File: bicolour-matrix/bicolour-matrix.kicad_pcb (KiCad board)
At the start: 2 copper layers, 136.8 x 33.5 mm, 52 parts, among them J1 Conn_01x04_Pin, J2 Conn_01x04_Pin, U1 HT16K33A-28SSOP, U2 HT16K33A-28SSOP, U3 HT16K33A-28SSOP, U4 HT16K33A-28SSOP

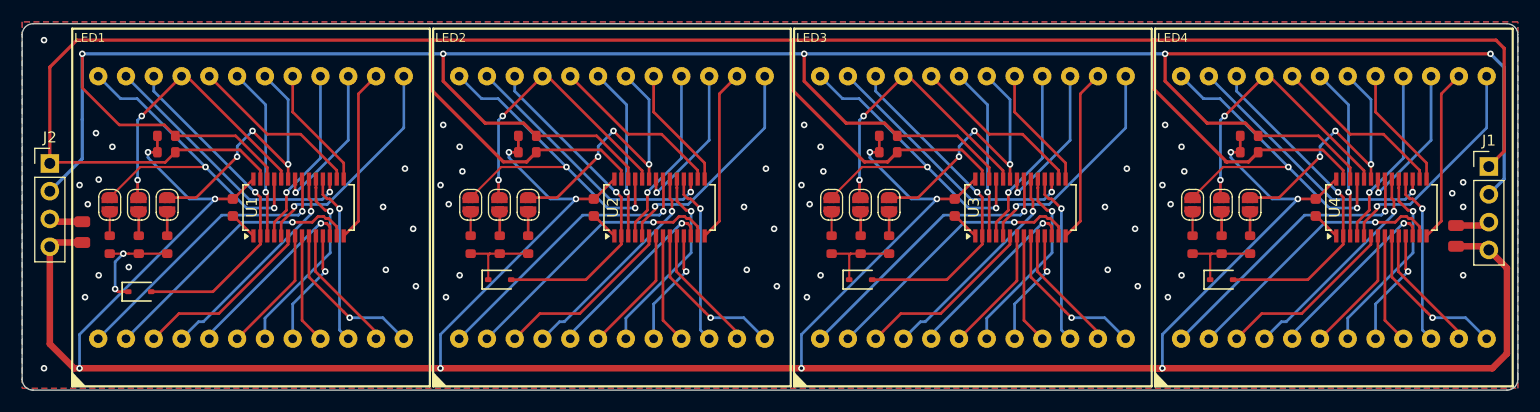
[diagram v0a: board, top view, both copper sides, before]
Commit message: feat: all changes
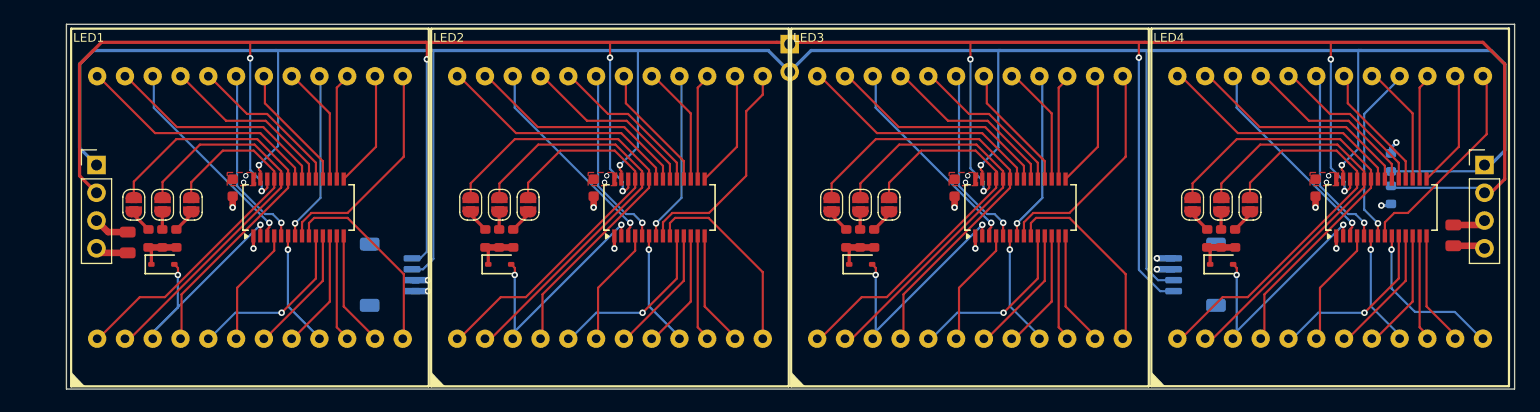
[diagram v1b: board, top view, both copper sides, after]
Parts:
- removed R12, R16, R17, R6, R7, R8: 4.7kΩ, PCM_JLCPCB:R_0603
- added J3: Conn_01x04_Socket, Connector_JST:JST_SH_SM04B-SRSS-TB_1x04-1MP_P1.00mm_Horizontal, B.Cu at (191.8, 94.0)
- added J4: Conn_01x04_Socket, Connector_JST:JST_SH_SM04B-SRSS-TB_1x04-1MP_P1.00mm_Horizontal, B.Cu at (118.2, 94.0)
- added J5: Conn_01x02_Socket, Connector_PinSocket_2.54mm:PinSocket_1x02_P2.54mm_Vertical, B.Cu at (154.7, 72.9)
- C2, C3, C4, C5: value 1uF -> 100nF
- R1, R2: value 4.7kΩ -> 10kΩ; footprint PCM_JLCPCB:R_0603 -> Resistor_SMD:R_0603_1608Metric; moved to B.Cu
- moved R1 79.1 mm to (209.7, 86.7), turned to 90 degrees
- moved R2 79.0 mm to (209.7, 83.7), turned to -90 degrees
- moved J2 4.27 mm to (91.3, 83.9)
- moved C6 4.26 mm to (94.2, 91.0)
- moved R11 3.59 mm to (96.0, 90.6)
- moved D1 3.27 mm to (97.4, 93.0)
- moved R9 2.23 mm to (97.3, 90.6)
- moved JP1 2.20 mm to (97.3, 87.5)
- moved JP2 2.20 mm to (100.0, 87.5)
- moved JP3 2.20 mm to (94.7, 87.5)
- moved C2 1.80 mm to (103.7, 86.0)
- moved C3 1.80 mm to (136.8, 86.0)
- moved C4 1.80 mm to (169.8, 86.0)
- moved C5 1.80 mm to (202.8, 86.0)
- moved R15 1.48 mm to (162.4, 90.6)
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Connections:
- net Net-(LED1-K8) renamed /Matrix 1/C7
- net Net-(LED2-K8) renamed /Matrix 2/C7
- net Net-(LED3-K8) renamed /Matrix 3/C7
- net Net-(LED4-K8) renamed /Matrix 4/C7
- D1 pad 2: Net-(LED1-K1) -> /Matrix 1/C0
- D2 pad 2: Net-(LED2-K1) -> /Matrix 2/C0
- D3 pad 2: Net-(LED3-K1) -> /Matrix 3/C0
- D4 pad 2: Net-(LED4-K1) -> /Matrix 4/C0
- J1 pad 1: /Matrix 1/SDA -> /SDA
- J1 pad 2: /Matrix 1/SCL -> /SCL
- J2 pad 1: /Matrix 1/SDA -> /SDA
- J2 pad 2: /Matrix 1/SCL -> /SCL
- JP1 pad 2: /Matrix 1/A1-1 -> /Matrix 1/R1
- JP10 pad 2: /Matrix 4/A2-1 -> /Matrix 4/R2
- JP11 pad 2: /Matrix 4/A1-1 -> /Matrix 4/R1
- JP12 pad 2: /Matrix 4/A0-1 -> /Matrix 4/R0
- JP2 pad 2: /Matrix 1/A0-1 -> /Matrix 1/R0
- JP3 pad 2: /Matrix 1/A2-1 -> /Matrix 1/R2
- JP4 pad 2: /Matrix 2/A2-1 -> /Matrix 2/R2
- JP5 pad 2: /Matrix 2/A1-1 -> /Matrix 2/R1
- JP6 pad 2: /Matrix 2/A0-1 -> /Matrix 2/R0
- JP7 pad 2: /Matrix 3/A2-1 -> /Matrix 3/R2
- JP8 pad 2: /Matrix 3/A1-1 -> /Matrix 3/R1
- JP9 pad 2: /Matrix 3/A0-1 -> /Matrix 3/R0
- LED1 pad 1: Net-(LED1-A9) -> /Matrix 1/R0
- LED1 pad 10: Net-(LED1-A15) -> /Matrix 1/R12
- LED1 pad 11: Net-(LED1-A16) -> /Matrix 1/R11
- LED1 pad 13: Net-(LED1-K4) -> /Matrix 1/C6
- LED1 pad 14: Net-(LED1-A8) -> /Matrix 1/R10
- LED1 pad 15: Net-(LED1-A7) -> /Matrix 1/R9
- LED1 pad 16: Net-(LED1-K3) -> /Matrix 1/C5
- LED1 pad 17: Net-(LED1-A6) -> /Matrix 1/R8
- LED1 pad 18: /Matrix 1/A0-1 -> /Matrix 1/R7
- LED1 pad 19: Net-(LED1-K2) -> /Matrix 1/C3
- LED1 pad 2: Net-(LED1-A10) -> /Matrix 1/R1
- LED1 pad 20: Net-(LED1-A4) -> /Matrix 1/R6
- LED1 pad 21: /Matrix 1/A1-1 -> /Matrix 1/R5
- LED1 pad 22: Net-(LED1-K1) -> /Matrix 1/C1
- LED1 pad 23: Net-(LED1-A2) -> /Matrix 1/R4
- LED1 pad 24: /Matrix 1/A2-1 -> /Matrix 1/R3
- LED1 pad 3: Net-(LED1-K5) -> /Matrix 1/C0
- LED1 pad 4: Net-(LED1-A11) -> /Matrix 1/R2
- LED1 pad 5: Net-(LED1-A12) -> /Matrix 1/R15
- LED1 pad 6: Net-(LED1-K6) -> /Matrix 1/C2
- LED1 pad 7: Net-(LED1-A13) -> /Matrix 1/R14
- LED1 pad 8: Net-(LED1-A14) -> /Matrix 1/R13
- LED1 pad 9: Net-(LED1-K7) -> /Matrix 1/C4
- LED2 pad 1: Net-(LED2-A9) -> /Matrix 2/R0
- LED2 pad 10: Net-(LED2-A15) -> /Matrix 2/R12
- LED2 pad 11: Net-(LED2-A16) -> /Matrix 2/R11
- LED2 pad 13: Net-(LED2-K4) -> /Matrix 2/C6
- LED2 pad 14: Net-(LED2-A8) -> /Matrix 2/R10
- LED2 pad 15: Net-(LED2-A7) -> /Matrix 2/R9
- LED2 pad 16: Net-(LED2-K3) -> /Matrix 2/C5
- LED2 pad 17: Net-(LED2-A6) -> /Matrix 2/R8
- LED2 pad 18: /Matrix 2/A0-1 -> /Matrix 2/R7
- LED2 pad 19: Net-(LED2-K2) -> /Matrix 2/C3
- LED2 pad 2: Net-(LED2-A10) -> /Matrix 2/R1
- LED2 pad 20: Net-(LED2-A4) -> /Matrix 2/R6
- LED2 pad 21: /Matrix 2/A1-1 -> /Matrix 2/R5
- LED2 pad 22: Net-(LED2-K1) -> /Matrix 2/C1
- LED2 pad 23: Net-(LED2-A2) -> /Matrix 2/R4
- LED2 pad 24: /Matrix 2/A2-1 -> /Matrix 2/R3
- LED2 pad 3: Net-(LED2-K5) -> /Matrix 2/C0
- LED2 pad 4: Net-(LED2-A11) -> /Matrix 2/R2
- LED2 pad 5: Net-(LED2-A12) -> /Matrix 2/R15
- LED2 pad 6: Net-(LED2-K6) -> /Matrix 2/C2
- LED2 pad 7: Net-(LED2-A13) -> /Matrix 2/R14
- LED2 pad 8: Net-(LED2-A14) -> /Matrix 2/R13
- LED2 pad 9: Net-(LED2-K7) -> /Matrix 2/C4
- LED3 pad 1: Net-(LED3-A9) -> /Matrix 3/R0
- LED3 pad 10: Net-(LED3-A15) -> /Matrix 3/R12
- LED3 pad 11: Net-(LED3-A16) -> /Matrix 3/R11
- LED3 pad 13: Net-(LED3-K4) -> /Matrix 3/C6
- LED3 pad 14: Net-(LED3-A8) -> /Matrix 3/R10
- LED3 pad 15: Net-(LED3-A7) -> /Matrix 3/R9
- LED3 pad 16: Net-(LED3-K3) -> /Matrix 3/C5
- LED3 pad 17: Net-(LED3-A6) -> /Matrix 3/R8
- LED3 pad 18: /Matrix 3/A0-1 -> /Matrix 3/R7
- LED3 pad 19: Net-(LED3-K2) -> /Matrix 3/C3
- LED3 pad 2: Net-(LED3-A10) -> /Matrix 3/R1
- LED3 pad 20: Net-(LED3-A4) -> /Matrix 3/R6
- LED3 pad 21: /Matrix 3/A1-1 -> /Matrix 3/R5
- LED3 pad 22: Net-(LED3-K1) -> /Matrix 3/C1
- LED3 pad 23: Net-(LED3-A2) -> /Matrix 3/R4
- LED3 pad 24: /Matrix 3/A2-1 -> /Matrix 3/R3
- LED3 pad 3: Net-(LED3-K5) -> /Matrix 3/C0
- LED3 pad 4: Net-(LED3-A11) -> /Matrix 3/R2
- LED3 pad 5: Net-(LED3-A12) -> /Matrix 3/R15
- LED3 pad 6: Net-(LED3-K6) -> /Matrix 3/C2
- LED3 pad 7: Net-(LED3-A13) -> /Matrix 3/R14
- LED3 pad 8: Net-(LED3-A14) -> /Matrix 3/R13
- LED3 pad 9: Net-(LED3-K7) -> /Matrix 3/C4
- LED4 pad 1: Net-(LED4-A9) -> /Matrix 4/R0
- LED4 pad 10: Net-(LED4-A15) -> /Matrix 4/R12
- LED4 pad 11: Net-(LED4-A16) -> /Matrix 4/R11
- LED4 pad 13: Net-(LED4-K4) -> /Matrix 4/C6
- LED4 pad 14: Net-(LED4-A8) -> /Matrix 4/R10
- LED4 pad 15: Net-(LED4-A7) -> /Matrix 4/R9
- LED4 pad 16: Net-(LED4-K3) -> /Matrix 4/C5
- LED4 pad 17: Net-(LED4-A6) -> /Matrix 4/R8
- LED4 pad 18: /Matrix 4/A0-1 -> /Matrix 4/R7
- LED4 pad 19: Net-(LED4-K2) -> /Matrix 4/C3
- LED4 pad 2: Net-(LED4-A10) -> /Matrix 4/R1
- LED4 pad 20: Net-(LED4-A4) -> /Matrix 4/R6
- LED4 pad 21: /Matrix 4/A1-1 -> /Matrix 4/R5
- LED4 pad 22: Net-(LED4-K1) -> /Matrix 4/C1
- LED4 pad 23: Net-(LED4-A2) -> /Matrix 4/R4
- LED4 pad 24: /Matrix 4/A2-1 -> /Matrix 4/R3
- LED4 pad 3: Net-(LED4-K5) -> /Matrix 4/C0
- LED4 pad 4: Net-(LED4-A11) -> /Matrix 4/R2
- LED4 pad 5: Net-(LED4-A12) -> /Matrix 4/R15
- LED4 pad 6: Net-(LED4-K6) -> /Matrix 4/C2
- LED4 pad 7: Net-(LED4-A13) -> /Matrix 4/R14
- LED4 pad 8: Net-(LED4-A14) -> /Matrix 4/R13
- LED4 pad 9: Net-(LED4-K7) -> /Matrix 4/C4
- R1 pad 2: /Matrix 1/SDA -> /SCL
- R2 pad 2: /Matrix 1/SCL -> /SDA
- U1 pad 10: Net-(LED1-A16) -> /Matrix 1/R15
- U1 pad 11: Net-(LED1-A14) -> /Matrix 1/R14
- U1 pad 12: Net-(LED1-A12) -> /Matrix 1/R13
- U1 pad 13: Net-(LED1-A10) -> /Matrix 1/R12
- U1 pad 14: Net-(LED1-A8) -> /Matrix 1/R11
- U1 pad 15: Net-(LED1-A6) -> /Matrix 1/R10
- U1 pad 16: Net-(LED1-A4) -> /Matrix 1/R9
- U1 pad 17: Net-(LED1-A2) -> /Matrix 1/R8
- U1 pad 18: Net-(LED1-A15) -> /Matrix 1/R7
- U1 pad 19: Net-(LED1-A13) -> /Matrix 1/R6
- U1 pad 2: Net-(LED1-K1) -> /Matrix 1/C0
- U1 pad 20: Net-(LED1-A11) -> /Matrix 1/R5
- U1 pad 21: Net-(LED1-A9) -> /Matrix 1/R4
- U1 pad 22: Net-(LED1-A7) -> /Matrix 1/R3
- U1 pad 23: /Matrix 1/A0-1 -> /Matrix 1/R2
- U1 pad 24: /Matrix 1/A1-1 -> /Matrix 1/R1
- U1 pad 25: /Matrix 1/A2-1 -> /Matrix 1/R0
- U1 pad 26: /Matrix 1/SCL -> /SCL
- U1 pad 27: /Matrix 1/SDA -> /SDA
- U1 pad 3: Net-(LED1-K2) -> /Matrix 1/C1
- U1 pad 4: Net-(LED1-K3) -> /Matrix 1/C2
- U1 pad 5: Net-(LED1-K4) -> /Matrix 1/C3
- U1 pad 6: Net-(LED1-K5) -> /Matrix 1/C4
- U1 pad 7: Net-(LED1-K6) -> /Matrix 1/C5
- U1 pad 8: Net-(LED1-K7) -> /Matrix 1/C6
- U2 pad 10: Net-(LED2-A16) -> /Matrix 2/R15
- U2 pad 11: Net-(LED2-A14) -> /Matrix 2/R14
- U2 pad 12: Net-(LED2-A12) -> /Matrix 2/R13
- U2 pad 13: Net-(LED2-A10) -> /Matrix 2/R12
- U2 pad 14: Net-(LED2-A8) -> /Matrix 2/R11
- U2 pad 15: Net-(LED2-A6) -> /Matrix 2/R10
- U2 pad 16: Net-(LED2-A4) -> /Matrix 2/R9
- U2 pad 17: Net-(LED2-A2) -> /Matrix 2/R8
- U2 pad 18: Net-(LED2-A15) -> /Matrix 2/R7
- U2 pad 19: Net-(LED2-A13) -> /Matrix 2/R6
- U2 pad 2: Net-(LED2-K1) -> /Matrix 2/C0
- U2 pad 20: Net-(LED2-A11) -> /Matrix 2/R5
- U2 pad 21: Net-(LED2-A9) -> /Matrix 2/R4
- U2 pad 22: Net-(LED2-A7) -> /Matrix 2/R3
- U2 pad 23: /Matrix 2/A0-1 -> /Matrix 2/R2
- U2 pad 24: /Matrix 2/A1-1 -> /Matrix 2/R1
- U2 pad 25: /Matrix 2/A2-1 -> /Matrix 2/R0
- U2 pad 26: /Matrix 1/SCL -> /SCL
- U2 pad 27: /Matrix 1/SDA -> /SDA
- U2 pad 3: Net-(LED2-K2) -> /Matrix 2/C1
- U2 pad 4: Net-(LED2-K3) -> /Matrix 2/C2
- U2 pad 5: Net-(LED2-K4) -> /Matrix 2/C3
- U2 pad 6: Net-(LED2-K5) -> /Matrix 2/C4
- U2 pad 7: Net-(LED2-K6) -> /Matrix 2/C5
- U2 pad 8: Net-(LED2-K7) -> /Matrix 2/C6
- U3 pad 10: Net-(LED3-A16) -> /Matrix 3/R15
- U3 pad 11: Net-(LED3-A14) -> /Matrix 3/R14
- U3 pad 12: Net-(LED3-A12) -> /Matrix 3/R13
- U3 pad 13: Net-(LED3-A10) -> /Matrix 3/R12
- U3 pad 14: Net-(LED3-A8) -> /Matrix 3/R11
- U3 pad 15: Net-(LED3-A6) -> /Matrix 3/R10
- U3 pad 16: Net-(LED3-A4) -> /Matrix 3/R9
- U3 pad 17: Net-(LED3-A2) -> /Matrix 3/R8
- U3 pad 18: Net-(LED3-A15) -> /Matrix 3/R7
- U3 pad 19: Net-(LED3-A13) -> /Matrix 3/R6
- U3 pad 2: Net-(LED3-K1) -> /Matrix 3/C0
- U3 pad 20: Net-(LED3-A11) -> /Matrix 3/R5
- U3 pad 21: Net-(LED3-A9) -> /Matrix 3/R4
- U3 pad 22: Net-(LED3-A7) -> /Matrix 3/R3
- U3 pad 23: /Matrix 3/A0-1 -> /Matrix 3/R2
- U3 pad 24: /Matrix 3/A1-1 -> /Matrix 3/R1
- U3 pad 25: /Matrix 3/A2-1 -> /Matrix 3/R0
- U3 pad 26: /Matrix 1/SCL -> /SCL
- U3 pad 27: /Matrix 1/SDA -> /SDA
- U3 pad 3: Net-(LED3-K2) -> /Matrix 3/C1
- U3 pad 4: Net-(LED3-K3) -> /Matrix 3/C2
- U3 pad 5: Net-(LED3-K4) -> /Matrix 3/C3
- U3 pad 6: Net-(LED3-K5) -> /Matrix 3/C4
- U3 pad 7: Net-(LED3-K6) -> /Matrix 3/C5
- U3 pad 8: Net-(LED3-K7) -> /Matrix 3/C6
- U4 pad 10: Net-(LED4-A16) -> /Matrix 4/R15
- U4 pad 11: Net-(LED4-A14) -> /Matrix 4/R14
- U4 pad 12: Net-(LED4-A12) -> /Matrix 4/R13
- U4 pad 13: Net-(LED4-A10) -> /Matrix 4/R12
- U4 pad 14: Net-(LED4-A8) -> /Matrix 4/R11
- U4 pad 15: Net-(LED4-A6) -> /Matrix 4/R10
- U4 pad 16: Net-(LED4-A4) -> /Matrix 4/R9
- U4 pad 17: Net-(LED4-A2) -> /Matrix 4/R8
- U4 pad 18: Net-(LED4-A15) -> /Matrix 4/R7
- U4 pad 19: Net-(LED4-A13) -> /Matrix 4/R6
- U4 pad 2: Net-(LED4-K1) -> /Matrix 4/C0
- U4 pad 20: Net-(LED4-A11) -> /Matrix 4/R5
- U4 pad 21: Net-(LED4-A9) -> /Matrix 4/R4
- U4 pad 22: Net-(LED4-A7) -> /Matrix 4/R3
- U4 pad 23: /Matrix 4/A0-1 -> /Matrix 4/R2
- U4 pad 24: /Matrix 4/A1-1 -> /Matrix 4/R1
- U4 pad 25: /Matrix 4/A2-1 -> /Matrix 4/R0
- U4 pad 26: /Matrix 1/SCL -> /SCL
- U4 pad 27: /Matrix 1/SDA -> /SDA
- U4 pad 3: Net-(LED4-K2) -> /Matrix 4/C1
- U4 pad 4: Net-(LED4-K3) -> /Matrix 4/C2
- U4 pad 5: Net-(LED4-K4) -> /Matrix 4/C3
- U4 pad 6: Net-(LED4-K5) -> /Matrix 4/C4
- U4 pad 7: Net-(LED4-K6) -> /Matrix 4/C5
- U4 pad 8: Net-(LED4-K7) -> /Matrix 4/C6
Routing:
- net VDD: track 302.3 -> 11.0 mm
- net /SCL: track 0.00 -> 274.3 mm, vias 0 -> 10
- net /SDA: track 0.00 -> 258.3 mm, vias 0 -> 4
- net /Matrix 1/SDA: track 255.4 -> 0.00 mm
- net /Matrix 1/SCL: track 251.6 -> 0.00 mm, vias 5 -> 0
- net /Matrix 2/R2: track 0.00 -> 40.0 mm
- net /Matrix 4/R2: track 0.00 -> 40.0 mm
- net /Matrix 3/R2: track 0.00 -> 40.0 mm
- net /Matrix 4/R1: track 0.00 -> 39.2 mm
- net /Matrix 2/R1: track 0.00 -> 39.2 mm
- net /Matrix 3/R1: track 0.00 -> 39.2 mm
- net /Matrix 1/R2: track 0.00 -> 37.9 mm
- net /Matrix 1/R1: track 0.00 -> 37.0 mm
- net /Matrix 3/R0: track 0.00 -> 36.6 mm
- net /Matrix 2/R0: track 0.00 -> 36.6 mm
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- added copper zone on In1.Cu, net GND
- added copper zone on F.Cu, net VDD
- added copper zone on In2.Cu, net VDD
- removed copper zone on B.Cu, net GND
- removed copper zone on F.Cu, net GND
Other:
- board size 136.8 x 33.5 mm -> 132.4 x 33.4 mm
- copper layers 2 -> 4
- board text added: "SDA SCL GND +5V"
- board text added: "pullups"
- board text removed: "GND"
- board text removed: "VDD"
